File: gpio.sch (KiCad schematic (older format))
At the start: 38 parts, among them J6 Pro Bus, J7 PMOD1, J8 PMOD, SW1 SW_Push, SW2 SW_Push, U15 TXB0108PWR, U16 TXB0108PWR

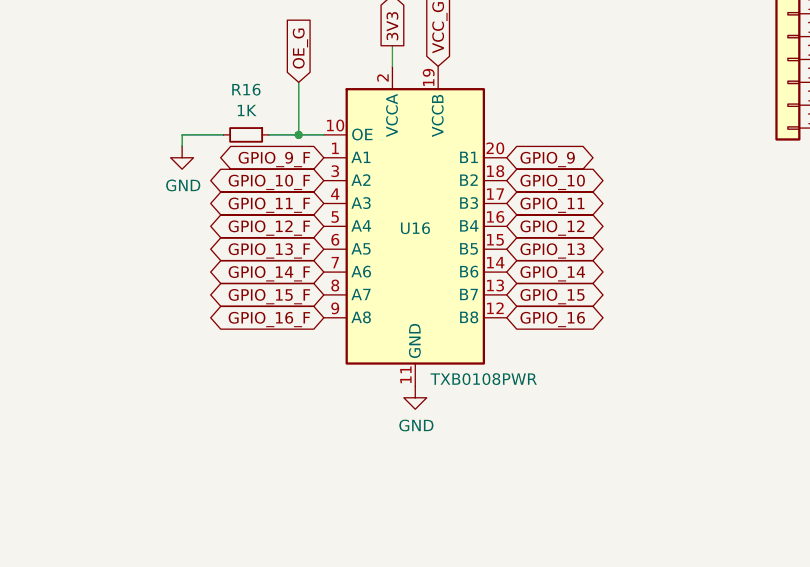
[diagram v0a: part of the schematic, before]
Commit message: mirror flipped the chips
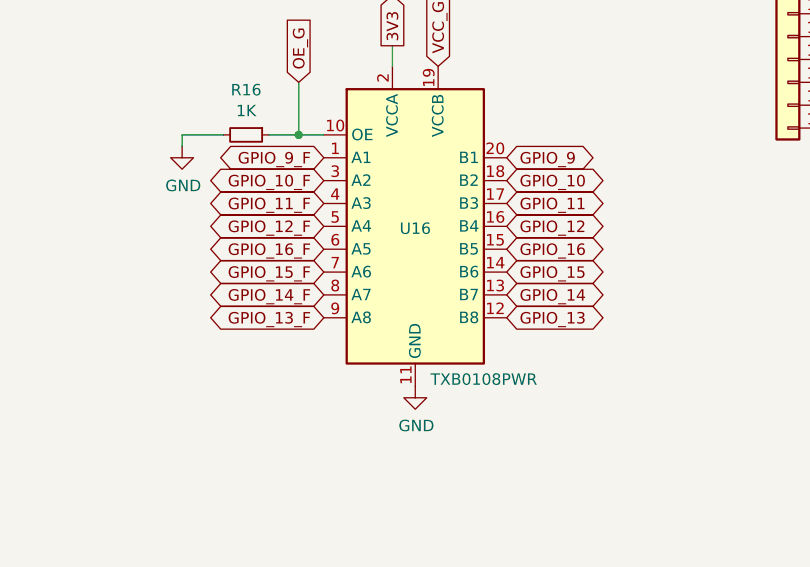
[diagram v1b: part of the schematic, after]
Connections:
- net GPIO_13: now also U16.12 (B8); no longer U16.15 (B5)
- net GPIO_13_F: now also U16.9 (A8); no longer U16.6 (A5)
- net GPIO_14: now also U16.13 (B7); no longer U16.14 (B6)
- net GPIO_14_F: now also U16.8 (A7); no longer U16.7 (A6)
- net GPIO_15: now also U16.14 (B6); no longer U16.13 (B7)
- net GPIO_15_F: now also U16.7 (A6); no longer U16.8 (A7)
- net GPIO_16: now also U16.15 (B5); no longer U16.12 (B8)
- net GPIO_16_F: now also U16.6 (A5); no longer U16.9 (A8)
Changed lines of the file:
@@
 Text GLabel 9040 2760 2    50   3State ~ 0
 GPIO_1
-Text GLabel 9040 5640 2    50   3State ~ 0
-GPIO_16
-Text GLabel 9040 5540 2    50   3State ~ 0
-GPIO_15
-Text GLabel 9040 5440 2    50   3State ~ 0
-GPIO_14
-Text GLabel 9040 5340 2    50   3State ~ 0
-GPIO_13
 Text GLabel 9040 5240 2    50   3State ~ 0
 GPIO_12
@@
 GPIO_1_F
 Text GLabel 8240 5640 0    50   3State ~ 0
-GPIO_16_F
-Text GLabel 8240 5540 0    50   3State ~ 0
-GPIO_15_F
-Text GLabel 8240 5440 0    50   3State ~ 0
-GPIO_14_F
-Text GLabel 8240 5340 0    50   3State ~ 0
 GPIO_13_F
 Text GLabel 8240 5240 0    50   3State ~ 0
@@
 Connection ~ 3230 1530
 Connection ~ 6090 1950
+Text GLabel 9040 5640 2    50   3State ~ 0
+GPIO_13
+Text GLabel 9040 5540 2    50   3State ~ 0
+GPIO_14
+Text GLabel 9040 5440 2    50   3State ~ 0
+GPIO_15
+Text GLabel 9040 5340 2    50   3State ~ 0
+GPIO_16
+Text GLabel 8240 5540 0    50   3State ~ 0
+GPIO_14_F
+Text GLabel 8240 5440 0    50   3State ~ 0
+GPIO_15_F
+Text GLabel 8240 5340 0    50   3State ~ 0
+GPIO_16_F
 $EndSCHEMATC
